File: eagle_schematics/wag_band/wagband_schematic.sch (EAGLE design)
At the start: 14 parts, among them U2 TLV1117-33CDCY

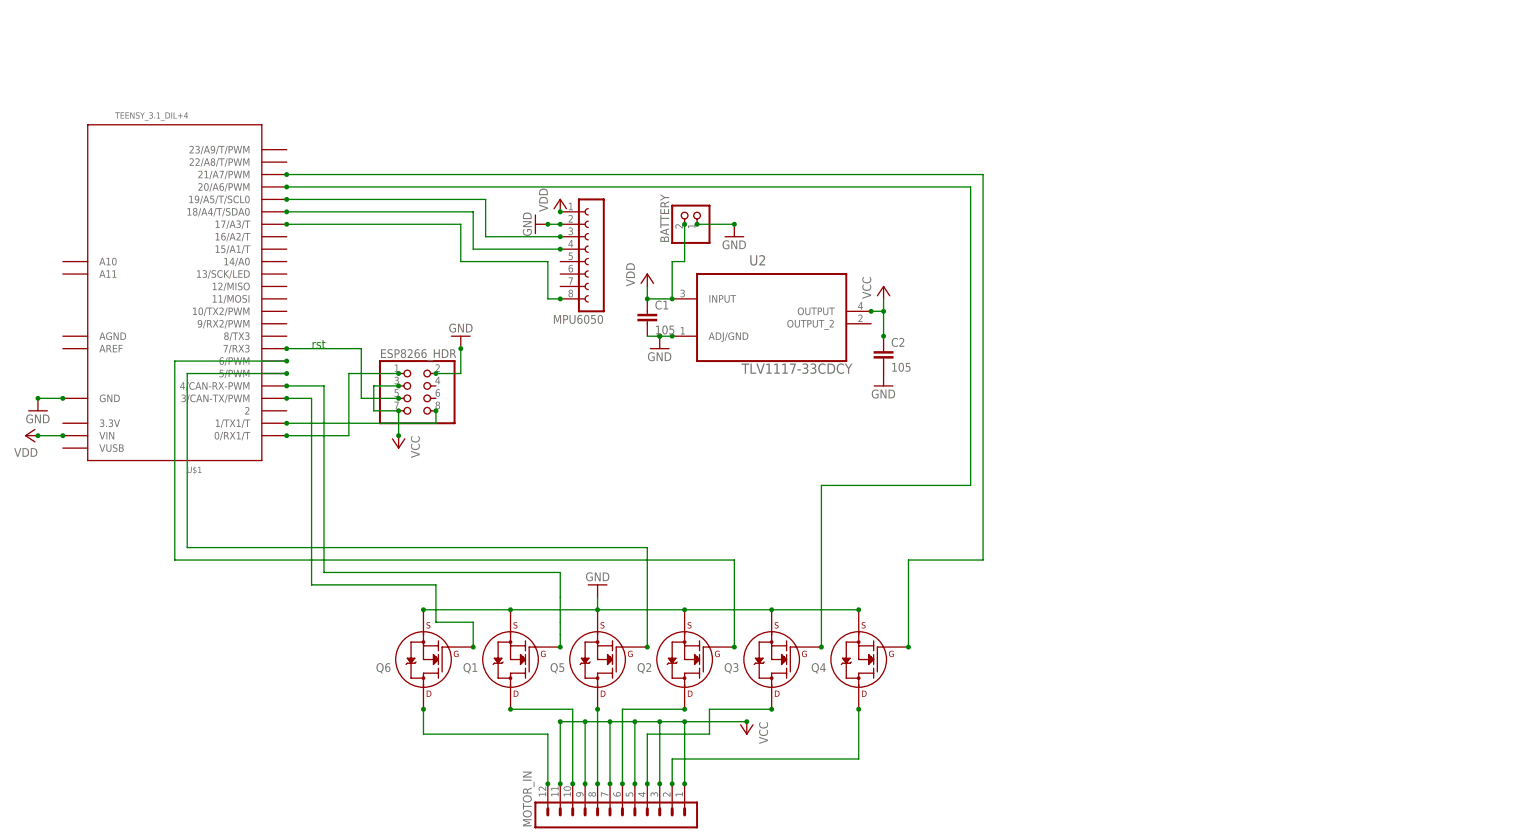
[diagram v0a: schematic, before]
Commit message: Added more parts for eagle
Finished PCBs
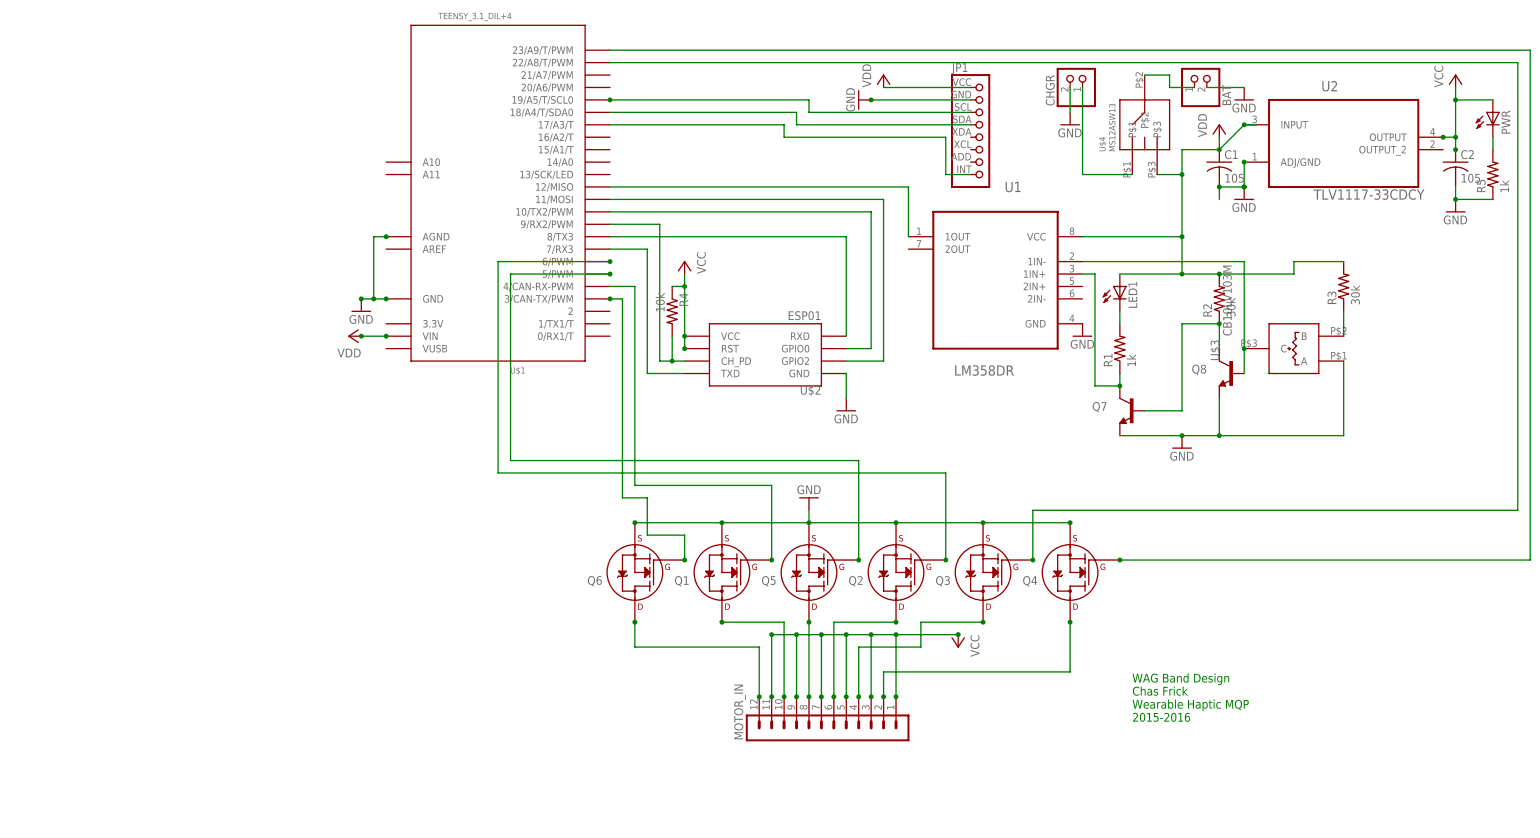
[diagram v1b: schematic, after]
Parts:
- removed BATTERY: (no value), adafruit:JST_2PIN-THM-RA
- removed ESP8266_HDR: (no value), pinhead:PINHD-2X4
- removed MPU6050: (no value), con-lsta:FE08-1
- added BAT, CHGR: (no value), adafruit:JST_2PIN-THM-RA
- added JP1: (no value), mqp_custom_parts:MPU6050_BREAKOUT
- added LED1, PWR: (no value), led:LED5MM
- added Q7, Q8: (no value), mqp_custom_parts:TRANSISTOR_NPNMMBT3904
- added R1, R5: 1k, resistor:R-US_R1206
- added R2, R3: 30k, resistor:R-US_R1206
- added R4: 10k, resistor:R-US_R1206
- added U$2: ESP01, esp8266modules:ESP01
- added U$3: CB10LV103M, mqp_custom_parts:CB10LV103M
- added U$4: MS12ASW13, mqp_custom_parts:MS12ASW13
- added U1: LM358DR, Texas Instruments_By_element14_Batch_1:LM358DR
- C1, C2: device rcl:C-EU025-024X044 -> resistor:C-USC0805K
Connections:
- new net N$12: U$1.8/TX3, U$2.RXD
- new net N$18: U$1.11/MOSI, U$2.GPIO2
- new net N$20: Q7.C, R1.1, U1.1IN+
- new net N$22: LED1.C, R1.2
- new net N$23: Q7.B, Q8.C, R2.1
- new net N$24: R4.2, U$1.9/RX2/PWM, U$2.CH_PD
- new net N$25: Q8.B, U$3.C, U1.1IN-
- new net N$26: U$1.12/MISO, U1.1OUT
- new net N$27: R3.1, U$3.B
- new net N$28: BAT.2, U$4.P$2
- new net N$29: CHGR.2, U$4.P$1
- net GND: now also BAT.1, CHGR.1, JP1.GND, Q7.E, Q8.E, R5.1, U$1.AGND, U$2.GND, U$3.A, U1.GND; no longer BATTERY.2, ESP8266_HDR.2, MPU6050.2
- net N$1: now also U$1.23/A9/T/PWM; no longer U$1.21/A7/PWM
- net N$17: now also JP1.SCL; no longer MPU6050.3
- net N$19: now also U$1.10/TX2/PWM, U$2.GPIO0; no longer ESP8266_HDR.8, U$1.1/TX1/T
- net N$21: now also PWR.C, R5.2; no longer ESP8266_HDR.5, U$1.7/RX3
- net N$3: now also U$1.22/A8/T/PWM; no longer U$1.20/A6/PWM
- net N$4: now also JP1.SDA; no longer MPU6050.4
- net N$7: now also U$1.7/RX3, U$2.TXD; no longer ESP8266_HDR.1, U$1.0/RX1/T
- net N$8: now also JP1.INT; no longer MPU6050.8
- net VCC: now also JP1.VCC, LED1.A, PWR.A, R2.2, R3.2, R4.1, U$2.RST, U$2.VCC, U$4.P$3, U1.VCC; no longer BATTERY.1, ESP8266_HDR.3, ESP8266_HDR.7, MPU6050.1
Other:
- note added: "WAG Band Design Chas Frick Wearable Haptic MQP 2015-2016"
- note removed: "rst"
- moved on the sheet: C1, C2, MOTOR_IN, Q1, Q2, Q3, Q4, Q5, Q6, U$1, U2
